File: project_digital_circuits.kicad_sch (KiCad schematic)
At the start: 82 parts, among them J1 PADS_to_solder, J2 Conn_01x06_Pin, J3 Conn_01x06_Pin, J4 PADS_to_solder, J5 PADS_to_solder, J6 PADS_to_solder, J7 PADS_to_solder, P1 USB_C_Plug_USB2.0, P2 XT30PW-F, Q1 Si4214, Q2 Si4214, Q3 Si4214, Q4 AO3400A, Q5 AO3400A, Q6 AO3400A, SW1 SW_Push, U1 TB6612FNG, U2 LTC4365DDB, U3 LMR33630ADDA, U4 MPU-6050, U5 VL53L0CXV0DH1, U6 FT234XD-T, U7 ESP32-S3-MINI-1

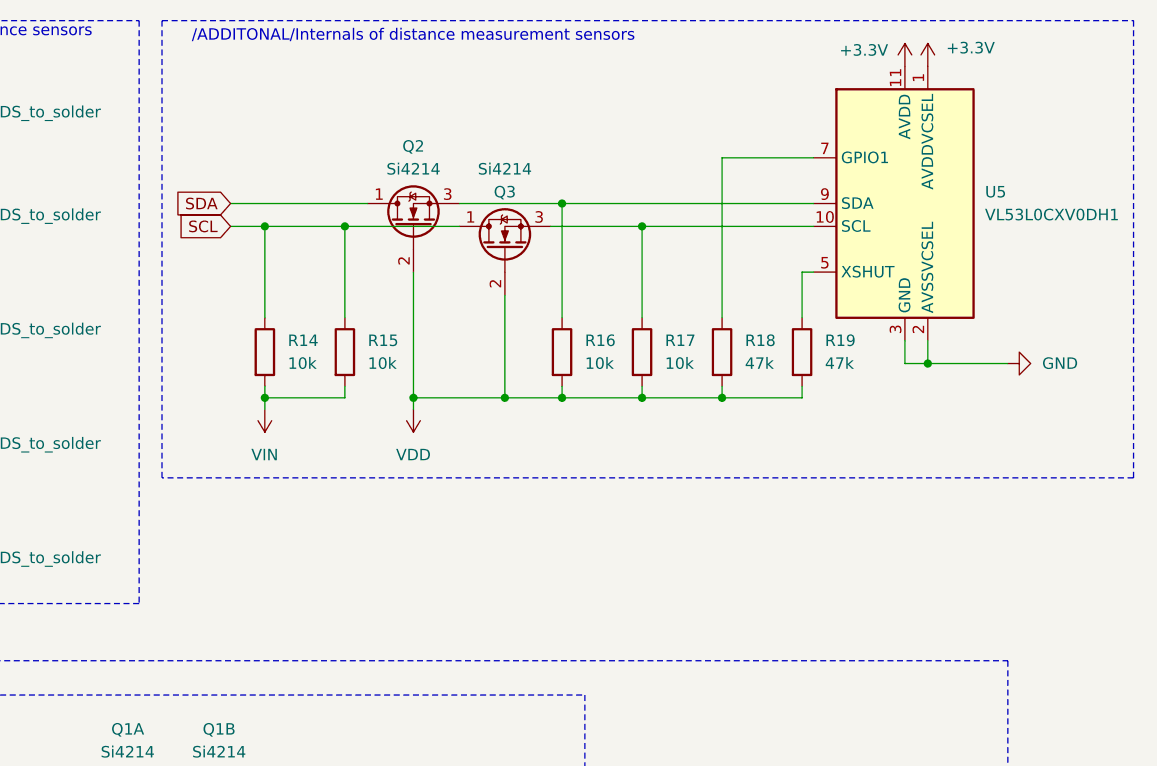
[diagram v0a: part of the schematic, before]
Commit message: final corrections of circuits
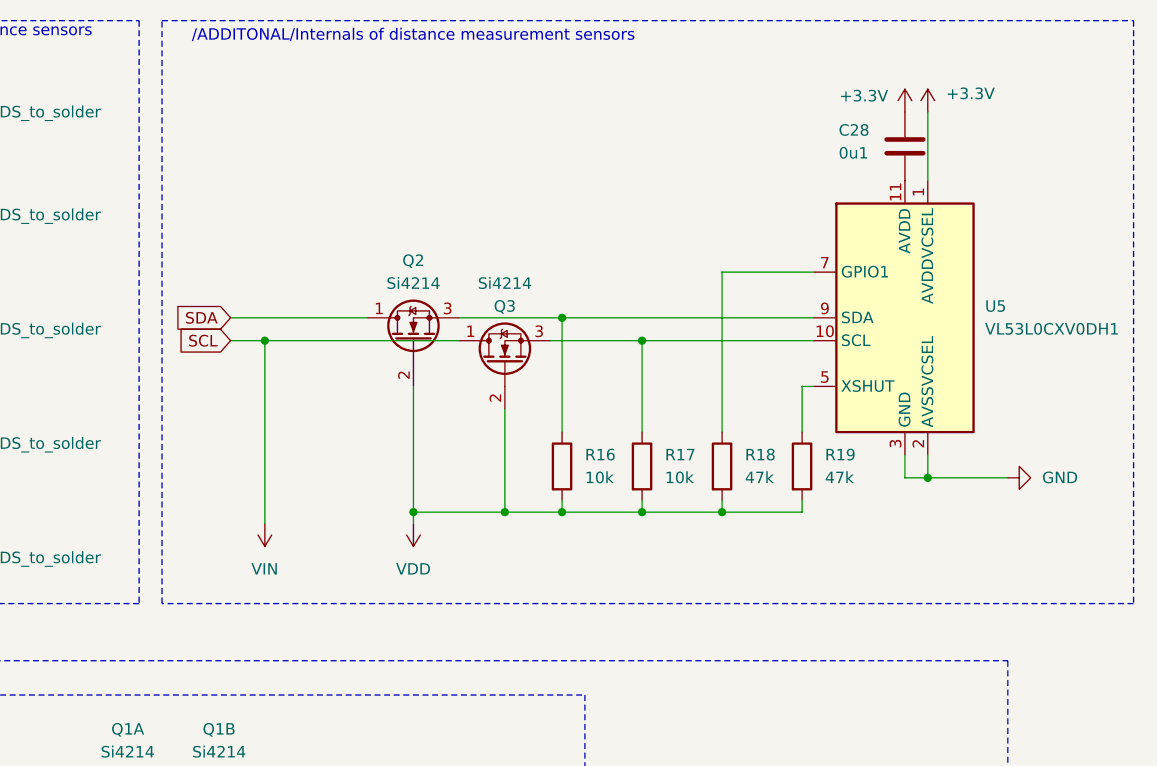
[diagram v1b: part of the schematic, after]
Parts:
- removed R14, R15: 10k, symbol Device:R
- added C28: 0u1, symbol Device:C
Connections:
- net SCL is gone; now on net VIN: Q3.1 (D)
- net +3.3V: now also C28.1; no longer U5.11 (AVDD)
- new net: C28.2, U5.11 (AVDD)
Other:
- moved on the sheet: Q2, Q3, R16, R17, R18, R19, U5

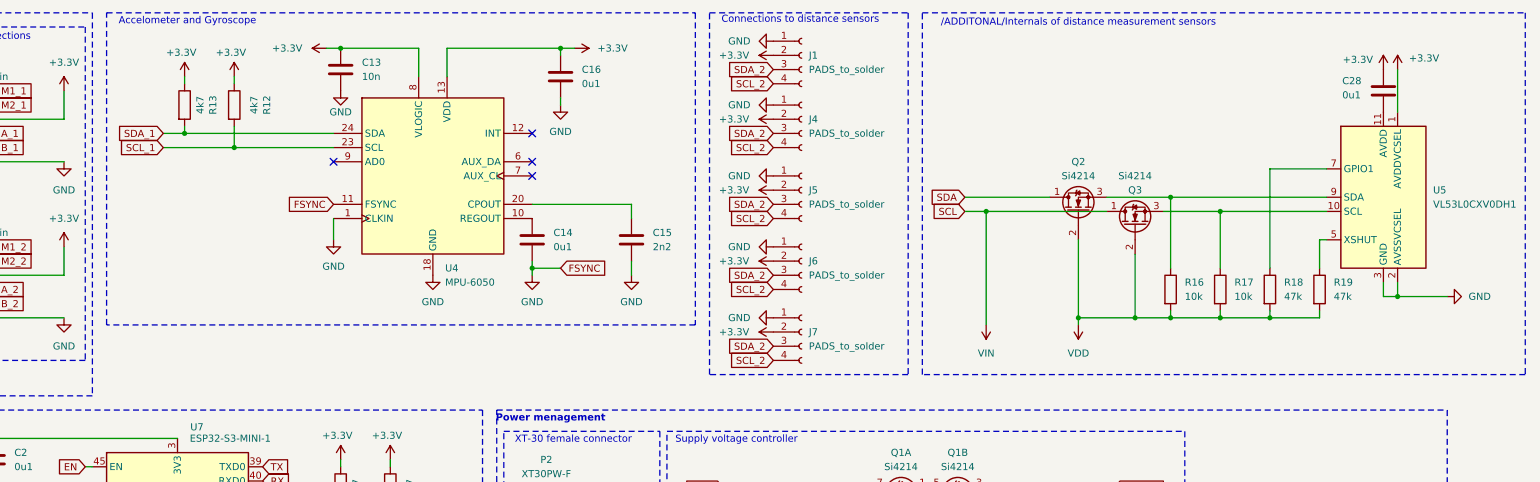
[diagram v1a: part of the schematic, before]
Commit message: final version of circuits
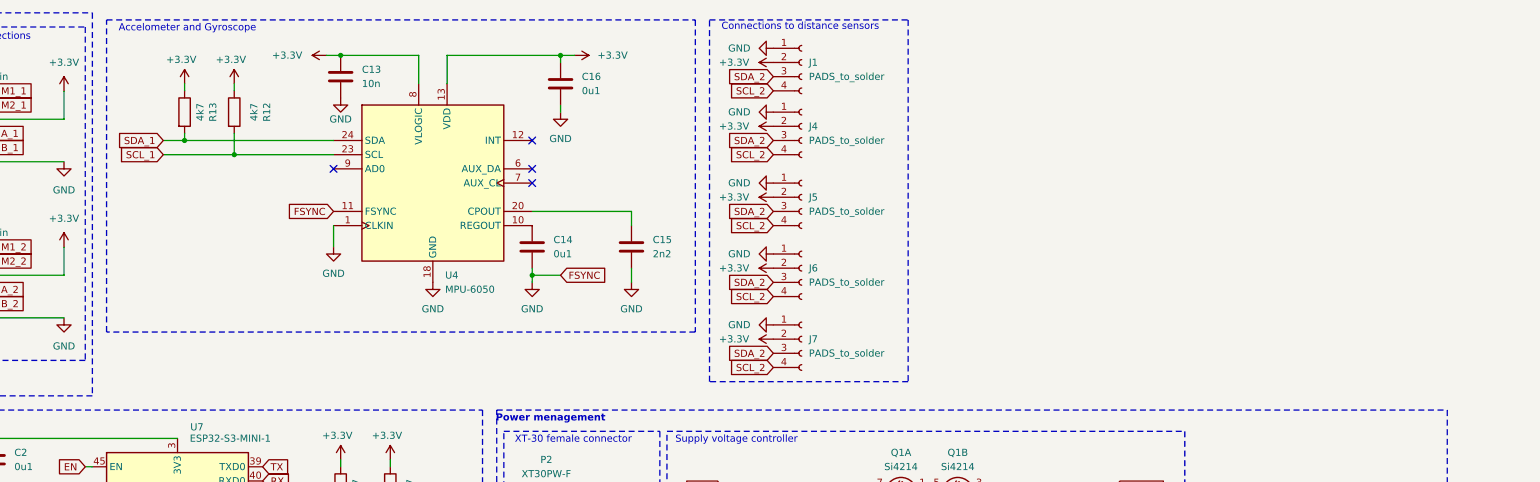
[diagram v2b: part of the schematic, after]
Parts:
- removed C28: 0u1, symbol Device:C
- removed Q2, Q3: Si4214, Package_TO_SOT_THT:TO-92_Inline, symbol Transistor_FET:BS108
- removed R16, R17: 10k, symbol Device:R
- removed R18, R19: 47k, symbol Device:R
- removed U5: VL53L0CXV0DH1, Sensor_Distance:ST_VL53L1x, symbol Sensor_Distance:VL53L0CXV0DH1
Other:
- note removed: "/ADDITONAL/Internals of distance measurement sensors"
- moved on the sheet: C13, C14, C15, C16, J1, J4, J5, J6, J7, R12, R13, U4
